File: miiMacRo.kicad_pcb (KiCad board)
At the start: 2 copper layers, 114.3 x 66.7 mm, 17 parts, among them SW1 SW_PUSH, SW10 SW_PUSH, SW11 SW_PUSH, SW12 Rotary_Encoder_Switch, SW2 SW_PUSH, SW3 SW_PUSH, SW4 SW_PUSH, SW5 SW_PUSH, SW6 SW_PUSH, SW7 SW_PUSH, SW8 SW_PUSH, SW9 SW_PUSH, U1 ProMicro

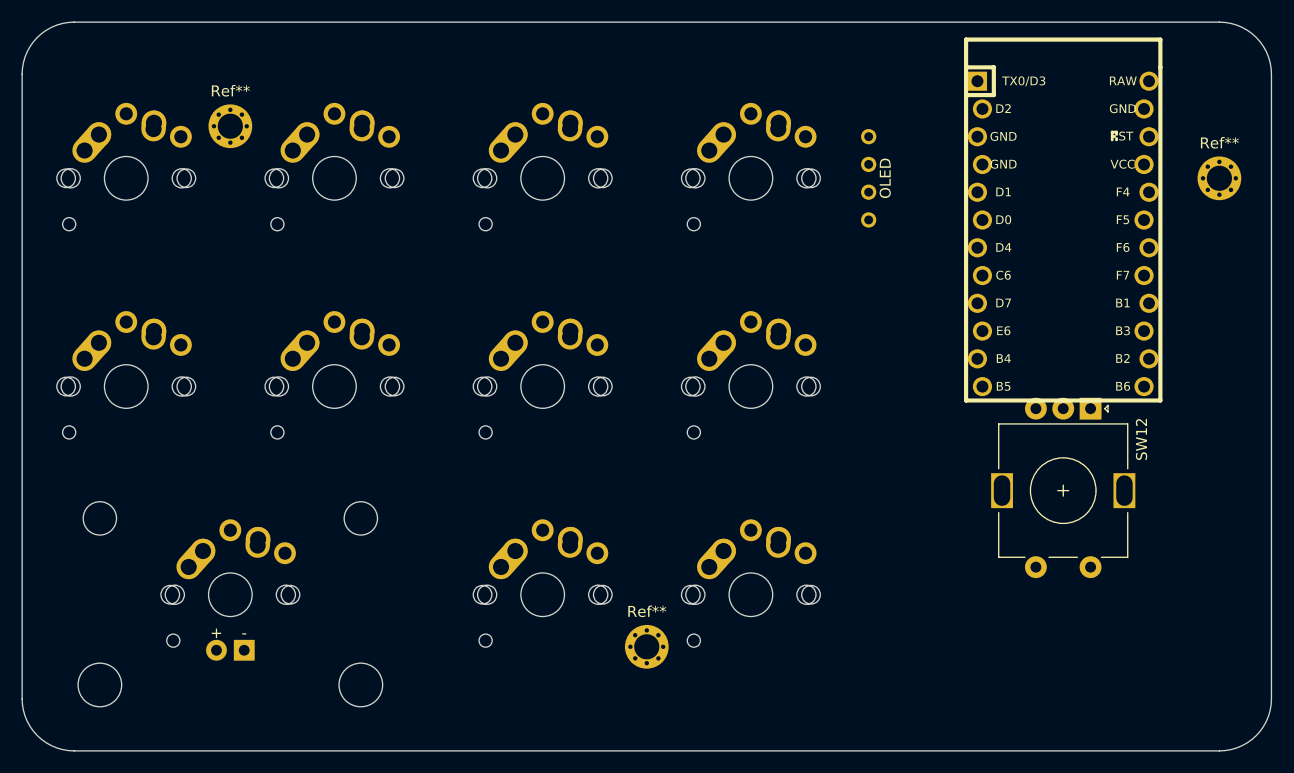
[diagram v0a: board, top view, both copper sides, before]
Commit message: first complete pcb
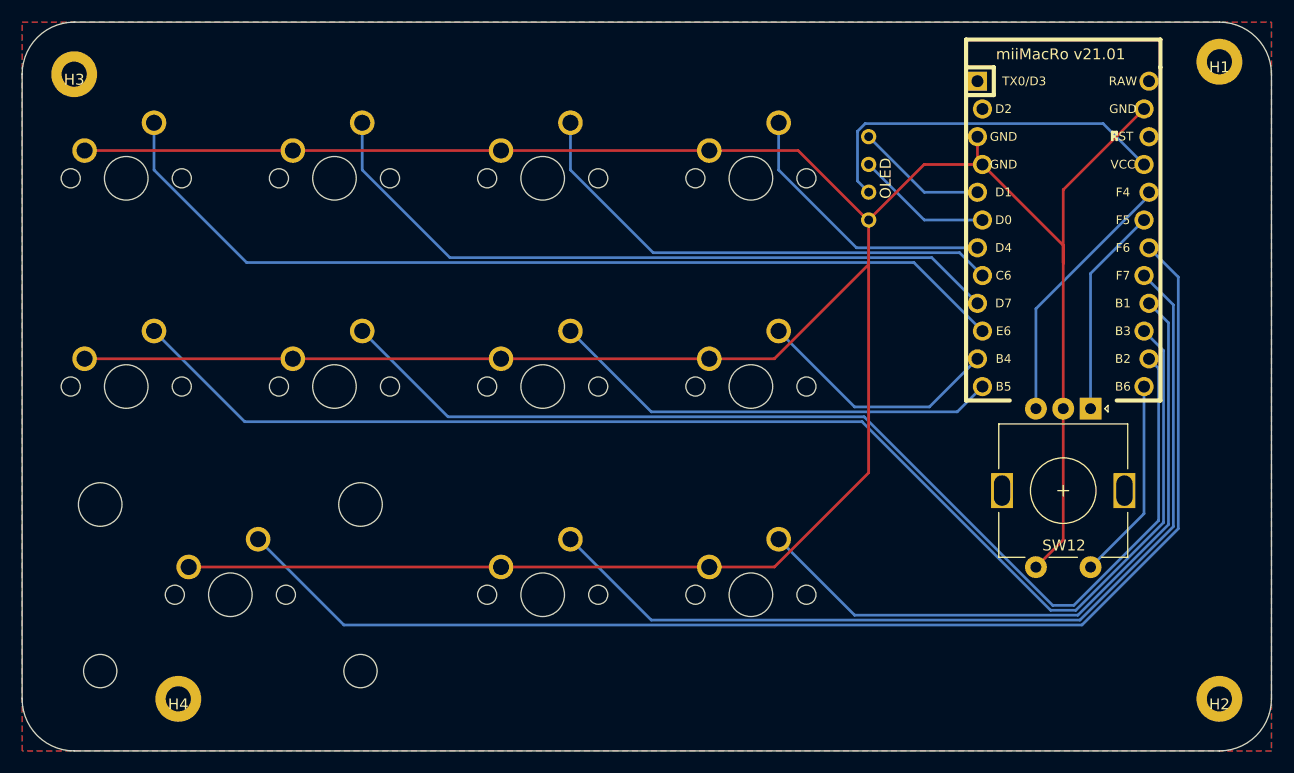
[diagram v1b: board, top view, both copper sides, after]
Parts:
- removed Ref** (x3): Val**, kbd:M2_HOLE_v3
- added H1: MountingHole, kbd:M2_Hole_TH, F.Cu at (181.0, 51.2)
- added H2: MountingHole, kbd:M2_Hole_TH, F.Cu at (181.0, 109.5)
- added H3: MountingHole, kbd:M2_Hole_TH, F.Cu at (76.2, 52.4)
- added H4: MountingHole, kbd:M2_Hole_TH, F.Cu at (85.7, 109.5)
- SW1: value SW_PUSH -> 1; footprint Keebio-Parts:MX-Alps-Choc-1U-NoLED -> MX_Only:MXOnly-1U-NoLED
- SW10: value SW_PUSH -> 8; footprint Keebio-Parts:MX-Alps-Choc-1U-NoLED -> MX_Only:MXOnly-1U-NoLED
- SW11: value SW_PUSH -> 0; footprint Keebio-Parts:MX-Alps-Choc-1U-NoLED -> MX_Only:MXOnly-1U-NoLED
- SW12: value Rotary_Encoder_Switch -> ROTARY
- SW2: value SW_PUSH -> 5; footprint Keebio-Parts:MX-Alps-Choc-1U-NoLED -> MX_Only:MXOnly-1U-NoLED
- SW3: value SW_PUSH -> ENTER; footprint Keebio-Parts:MX-Alps-Choc-2U -> MX_Only:MXOnly-2U-ReversedStabilizers-NoLED
- SW4: value SW_PUSH -> 2; footprint Keebio-Parts:MX-Alps-Choc-1U-NoLED -> MX_Only:MXOnly-1U-NoLED
- SW5: value SW_PUSH -> 6; footprint Keebio-Parts:MX-Alps-Choc-1U-NoLED -> MX_Only:MXOnly-1U-NoLED
- SW6: value SW_PUSH -> 3; footprint Keebio-Parts:MX-Alps-Choc-1U-NoLED -> MX_Only:MXOnly-1U-NoLED
- SW7: value SW_PUSH -> 7; footprint Keebio-Parts:MX-Alps-Choc-1U-NoLED -> MX_Only:MXOnly-1U-NoLED
- SW8: value SW_PUSH -> 9; footprint Keebio-Parts:MX-Alps-Choc-1U-NoLED -> MX_Only:MXOnly-1U-NoLED
- SW9: value SW_PUSH -> 4; footprint Keebio-Parts:MX-Alps-Choc-1U-NoLED -> MX_Only:MXOnly-1U-NoLED
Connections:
- OL1 pad 3: (no net) -> +5V
- SW1 pad 2: Net-(SW1-Pad2) -> E6
- SW10 pad 2: Net-(SW10-Pad2) -> B4
- SW11 pad 2: Net-(SW11-Pad2) -> B1
- SW12 pad A: (no net) -> F5
- SW12 pad B: (no net) -> F4
- SW12 pad S1: (no net) -> GND
- SW12 pad S2: GND -> B6
- SW2 pad 2: Net-(SW2-Pad2) -> B3
- SW3 pad 2: Net-(SW3-Pad2) -> F6
- SW4 pad 2: Net-(SW4-Pad2) -> D7
- SW5 pad 2: Net-(SW5-Pad2) -> B2
- SW6 pad 2: Net-(SW6-Pad2) -> C6
- SW7 pad 2: Net-(SW7-Pad2) -> B5
- SW8 pad 2: Net-(SW8-Pad2) -> F7
- SW9 pad 2: Net-(SW9-Pad2) -> D4
- U1 pad 10: (no net) -> E6
- U1 pad 11: (no net) -> B4
- U1 pad 12: (no net) -> B5
- U1 pad 13: (no net) -> B6
- U1 pad 14: (no net) -> B2
- U1 pad 15: (no net) -> B3
- U1 pad 16: (no net) -> B1
- U1 pad 17: (no net) -> F7
- U1 pad 18: (no net) -> F6
- U1 pad 19: (no net) -> F5
- U1 pad 20: (no net) -> F4
- U1 pad 21: (no net) -> +5V
- U1 pad 7: (no net) -> D4
- U1 pad 8: (no net) -> C6
- U1 pad 9: (no net) -> D7
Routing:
- net GND: track 0.00 -> 312.1 mm
- net B3: track 0.00 -> 124.5 mm
- net F6: track 0.00 -> 117.9 mm
- net B2: track 0.00 -> 101.6 mm
- net E6: track 0.00 -> 86.2 mm
- net F7: track 0.00 -> 85.8 mm
- net D7: track 0.00 -> 65.7 mm
- net B1: track 0.00 -> 63.0 mm
- net C6: track 0.00 -> 46.0 mm
- net B5: track 0.00 -> 41.7 mm
- net +5V: track 0.00 -> 34.1 mm
- net D4: track 0.00 -> 25.5 mm
- net F4: track 0.00 -> 24.1 mm
- net B4: track 0.00 -> 22.9 mm
- net F5: track 0.00 -> 19.3 mm
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- added copper zone on B.Cu, net (none)
- added copper zone on F.Cu, net (none)
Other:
- board text added: "miiMacRo v21.01"
